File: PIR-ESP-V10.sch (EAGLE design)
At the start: 13 parts

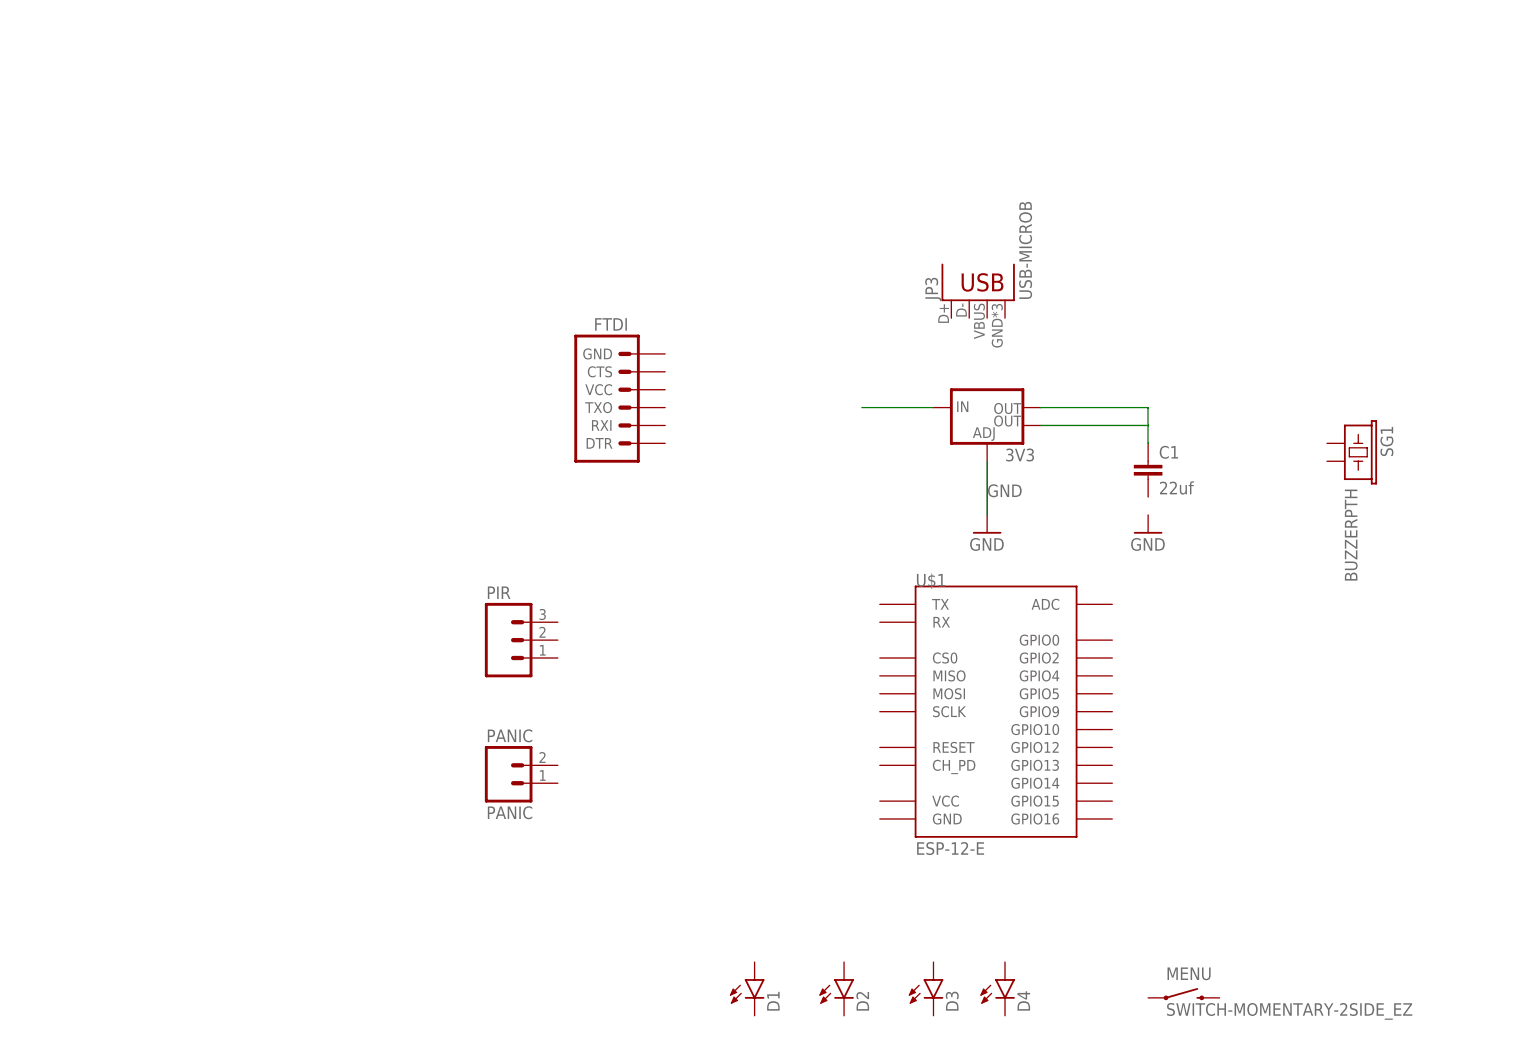
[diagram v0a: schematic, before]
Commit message: add wires
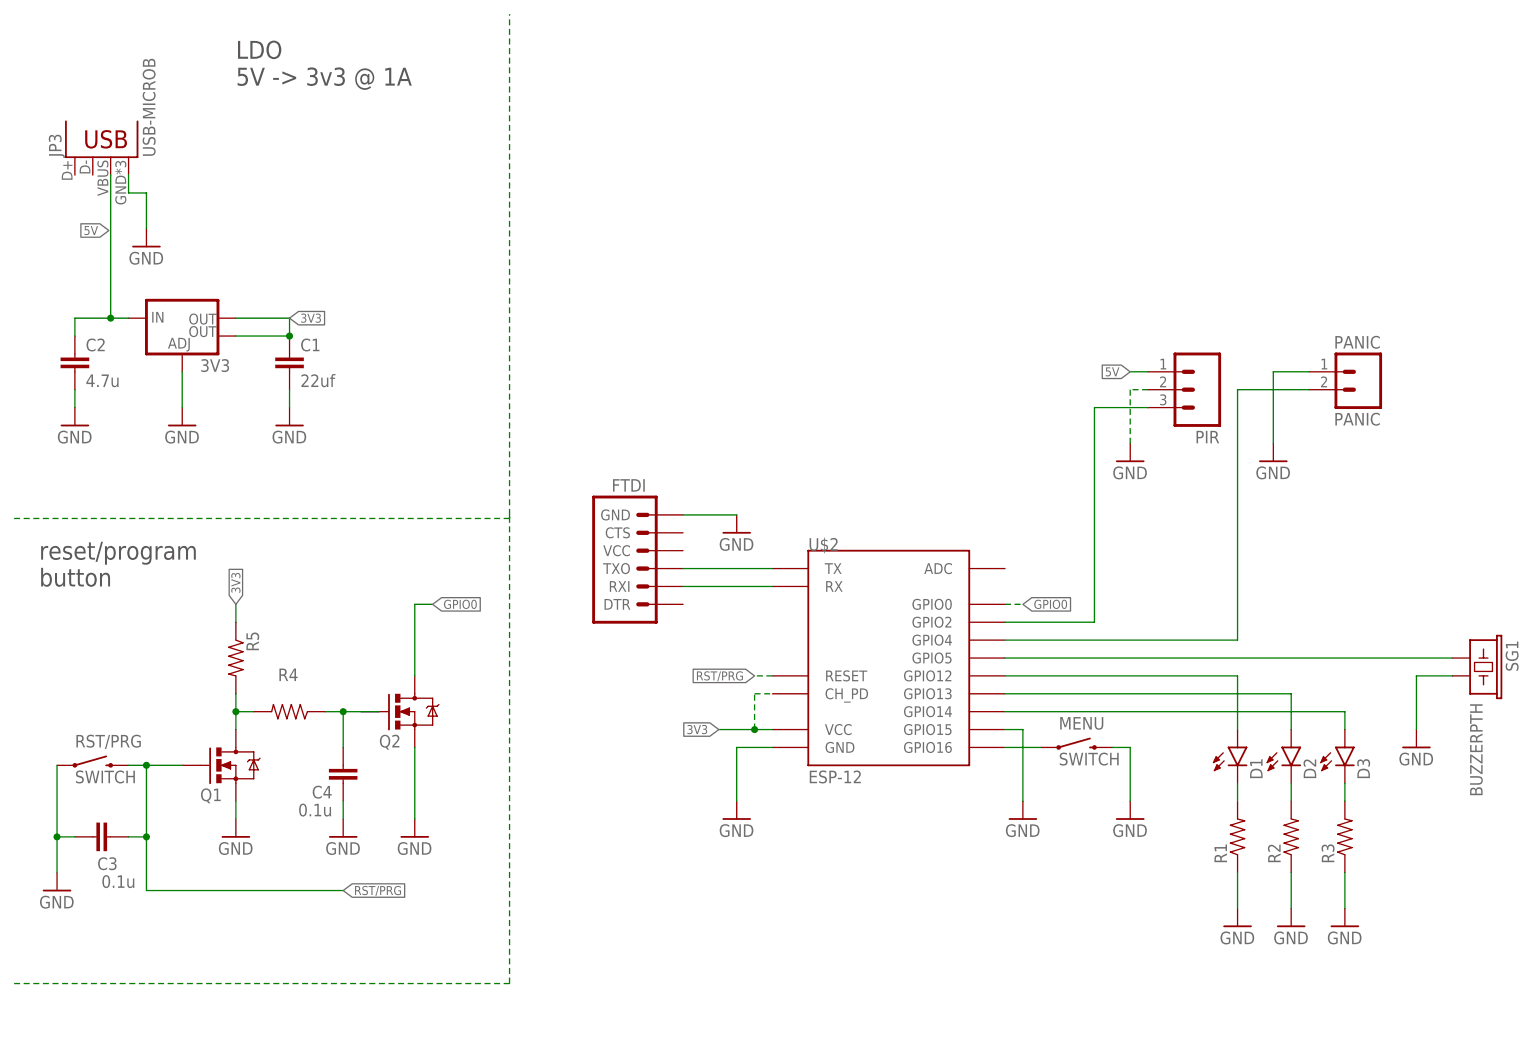
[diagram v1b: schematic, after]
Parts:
- removed D4: (no value), SparkFun-LED:LED5MM
- removed U$1: ESP-12-E, esp8266modules:ESP-12-E
- added C2: 4.7u, SparkFun-Passives:CAP1206
- added C3, C4: 0.1u, SparkFun-Passives:CAP1206
- added Q1, Q2: 200mA/50V, SparkFun-DiscreteSemi:MOSFET-NCHANNELBSS138
- added R1, R2, R3, R4, R5: (no value), SparkFun-Passives:RESISTOR1206
- added RST/PRG: SWITCH, SparkFun-Electromechanical:SWITCH-MOMENTARY-2SIDE_EZ
- added U$2: ESP-12, esp8266modules:ESP-12
- MENU: value SWITCH-MOMENTARY-2SIDE_EZ -> SWITCH
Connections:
- new net 3V3: 3V3.OUT, 3V3.OUT@1, C1.1, R5.1, U$2.CH_PD, U$2.VCC
- new net 5V: 3V3.IN, C2.1, JP3.VBUS, PIR.1
- new net GPIO0: Q2.D, U$2.GPIO0
- new net N$1: D1.A, U$2.GPIO12
- new net N$10: D2.A, U$2.GPIO13
- new net N$11: D3.A, U$2.GPIO14
- new net N$12: PIR.3, U$2.GPIO2
- new net N$14: C4.2, Q2.G, R4.1
- new net N$16: Q1.D, R4.2, R5.2
- new net N$5: FTDI.RXI, U$2.RX
- new net N$6: D1.C, R1.2
- new net N$7: D2.C, R2.2
- new net N$8: D3.C, R3.2
- new net N$9: PANIC.2, U$2.GPIO4
- new net RST/PRG: C3.2, Q1.G, RST/PRG.2, U$2.RESET
- net GND: now also C1.2, C2.2, C3.1, C4.1, FTDI.GND, JP3.GND, MENU.2, PANIC.1, PIR.2, Q1.S, Q2.S, R1.1, R2.1, R3.1, RST/PRG.1, SG1.2, U$2.GND, U$2.GPIO15
- net N$2: now also SG1.1, U$2.GPIO5; no longer 3V3.OUT@1
- net N$3: now also FTDI.TXO, U$2.TX; no longer 3V3.OUT, C1.1
- net N$4: now also MENU.1, U$2.GPIO16; no longer 3V3.IN
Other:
- note added: "LDO 5V -> 3v3 @ 1A"
- note added: "reset/program button"
- moved on the sheet: 3V3, C1, D1, D2, D3, FTDI, JP3, MENU, PANIC, PIR, SG1
